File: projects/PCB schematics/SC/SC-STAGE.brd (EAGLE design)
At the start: 160 x 100 mm, 0 parts

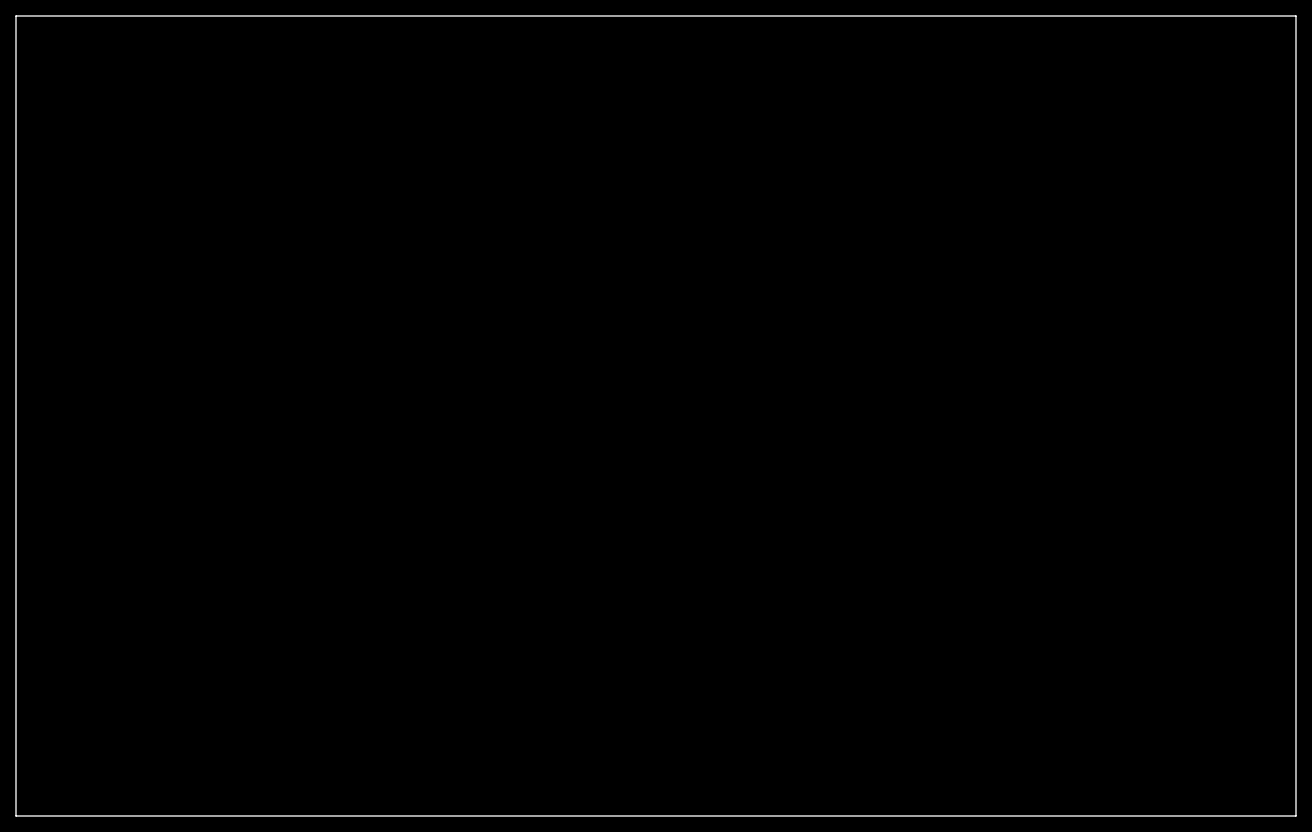
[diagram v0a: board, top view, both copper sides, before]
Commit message: SC - Stage initial placement.
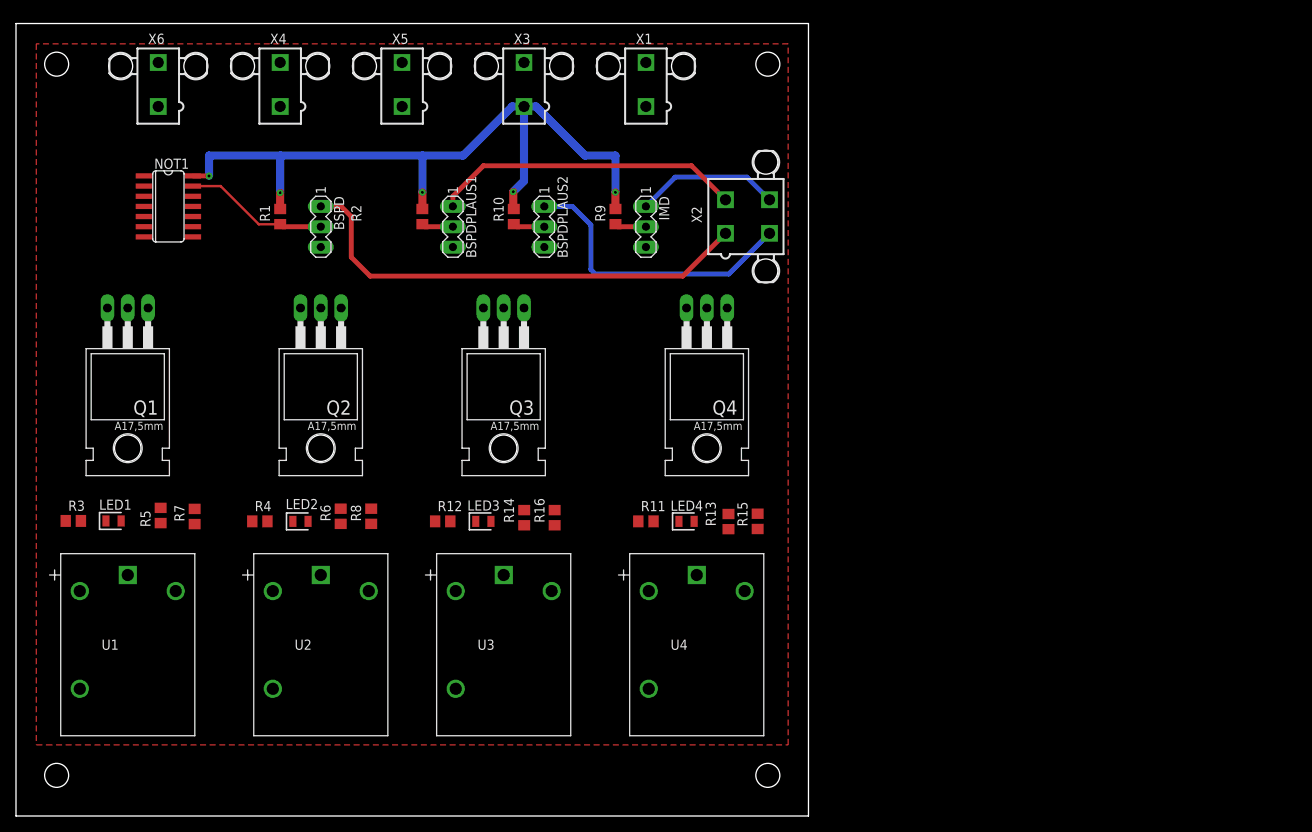
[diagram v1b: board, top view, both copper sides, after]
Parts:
- added BSPD, BSPDPLAUS1, BSPDPLAUS2, IMD: (no value), con-lstb:MA03-1
- added LED1, LED2, LED3, LED4: 150080VS75000, 150080VS75000:LEDC2012X80N
- added NOT1: 74LS19D, 74xx-us:SO14
- added Q1, Q2, Q3, Q4: IRLZ44Z, transistor-power:TO220BH
- added R1, R10, R11, R12, R2, R3, R4, R9: (no value), rcl:R0805
- added R13, R14, R5, R6: 47k, rcl:R0805
- added R15, R16, R7, R8: 100, rcl:R0805
- added U1, U2, U3, U4: G5LE-1A-E-DC12, IowaFormula:G5LE-1A-E-DC12
- added X1, X3, X4, X5, X6: 5566-2, con-molex:5566-2
- added X2: 5566-4, con-molex:5566-4
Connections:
- new net +12V: U1.5, U2.5, U3.5, U4.5
- new net +12V-ISO: X1.1, X1.2
- new net BSPDFAULT_LED: BSPD.1, X2.1
- new net BSPDPLAUS1_LED: BSPDPLAUS1.1, X2.2
- new net BSPDPLAUS2_LED: BSPDPLAUS2.1, X2.3
- new net GND: BSPD.3, BSPDPLAUS1.3, BSPDPLAUS2.3, IMD.3, NOT1.7, Q1.S, Q2.S, Q3.S, Q4.S, R11.1, R12.1, R13.1, R14.1, R3.1, R4.1, R5.1, R6.1, X5.1, X5.2
- new net IMDFAULT_LED: IMD.1, X2.4
- new net LED4: LED4.1, R11.2
- new net N$1: Q1.G, R7.2
- new net N$10: U3.1, U4.3
- new net N$105105: BSPD.2, NOT1.13, R1.1
- new net N$11552: BSPDPLAUS1.2, NOT1.11, R2.1
- new net N$14: Q4.G, R15.2
- new net N$15: LED4.2, NOT1.2, R13.2, R15.1
- new net N$17: Q4.D, U4.2
- new net N$18: Q3.G, R16.2
- new net N$19: LED3.2, NOT1.8, R14.2, R16.1
- new net N$2: LED1.2, NOT1.12, R5.2, R7.1
- new net N$20: LED3.1, R12.2
- new net N$21: Q3.D, U3.2
- new net N$3: LED1.1, R3.2
- new net N$38: U2.1, U3.3
- new net N$4: Q1.D, U1.2
- new net N$5: Q2.G, R8.2
- new net N$6: LED2.2, NOT1.10, R6.2, R8.1
- new net N$626: BSPDPLAUS2.2, NOT1.9, R10.1
- new net N$7: LED2.1, R4.2
- new net N$8: Q2.D, U2.2
- new net N$9: U1.1, U2.3
- new net N$9581: IMD.2, NOT1.1, R9.1
- new net SC+: U1.3, X4.1, X4.2
- new net SC-: U4.1, X6.1, X6.2
- new net VCC: NOT1.14, R1.2, R10.2, R2.2, R9.2, X3.1, X3.2
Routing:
- net VCC: track 0.00 -> 93.8 mm, vias 0 -> 5
- net BSPDFAULT_LED: track 0.00 -> 59.4 mm
- net BSPDPLAUS1_LED: track 0.00 -> 38.7 mm
- net BSPDPLAUS2_LED: track 0.00 -> 37.0 mm
- net IMDFAULT_LED: track 0.00 -> 18.1 mm
- net N$105105: track 0.00 -> 18.1 mm
- net N$626: track 0.00 -> 3.94 mm
- net N$11552: track 0.00 -> 3.94 mm
- net N$9581: track 0.00 -> 3.94 mm
- added copper zone on layer 1, net GND
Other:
- board size 160 x 100 mm -> 99.1 x 99.1 mm
